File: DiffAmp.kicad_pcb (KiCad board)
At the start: 2 copper layers, 99.7 x 35.6 mm, 111 parts, among them J1 USB_OTG, J2 Screw_Terminal_1x03, J3 Conn_01x02, J4 Conn_01x02, J5 Conn_01x02, U1 SF_IHXXXXS, U2 TPS7A49, U3 TPS7A30, U4 OPA189, U5 AD8421, U6 OPA189, U7 OPA189

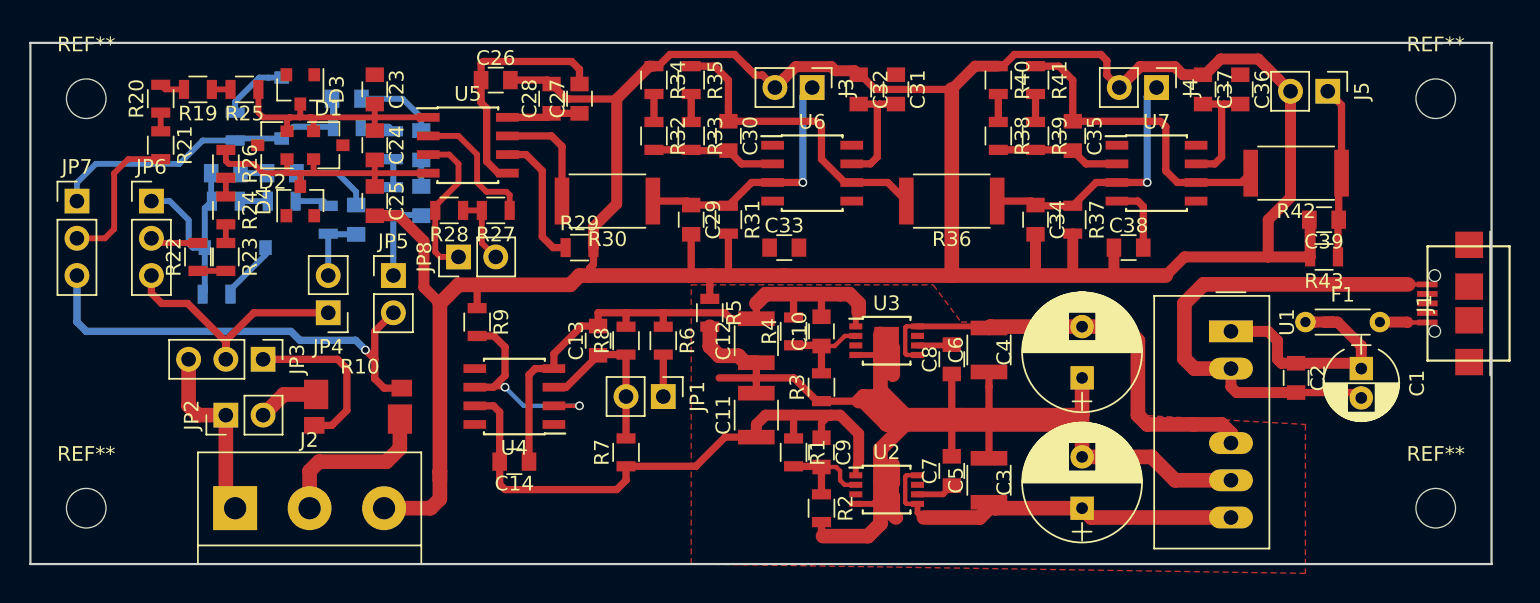
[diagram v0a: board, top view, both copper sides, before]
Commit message: Layout Completed
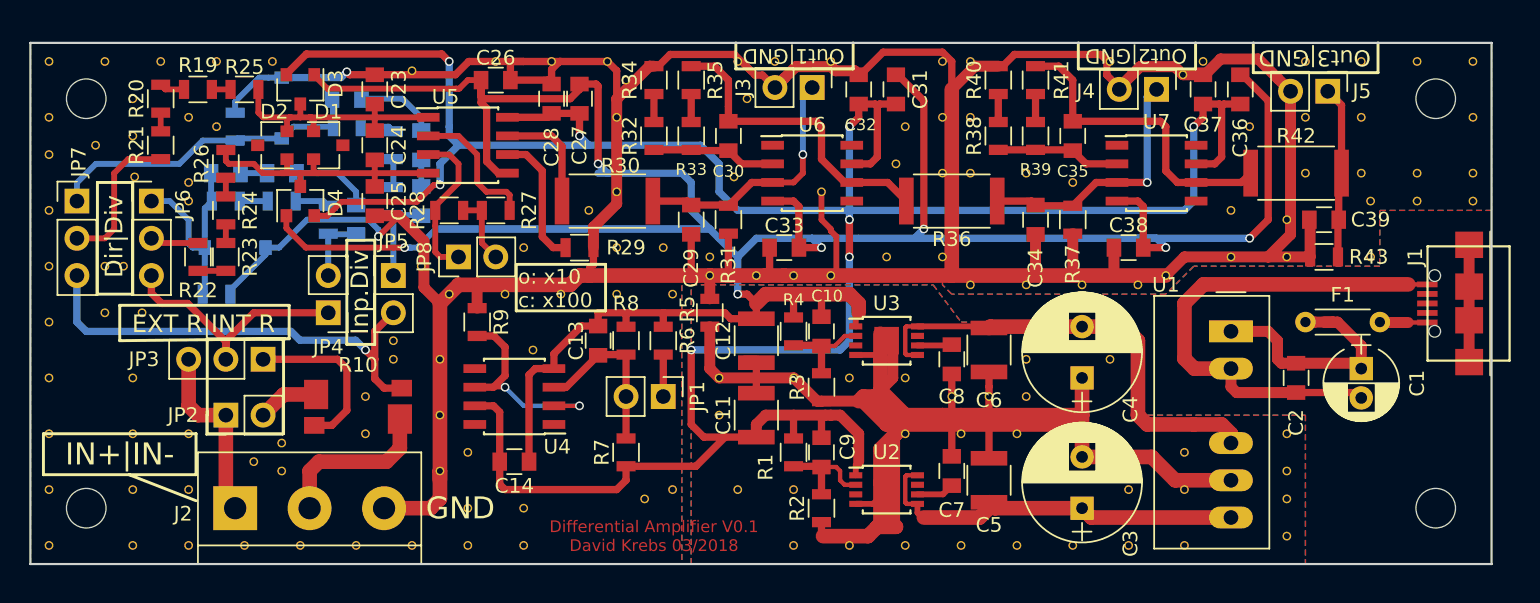
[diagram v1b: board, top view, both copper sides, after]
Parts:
- added ?: , DiffAmp:VIA-0.6mm, F.Cu at (119.8, 68.8)
- added ?: , DiffAmp:VIA-0.6mm, F.Cu at (76.8, 74.9)
- added ?: , DiffAmp:VIA-0.6mm, F.Cu at (162.6, 64.8)
- added ?: , DiffAmp:VIA-0.6mm, F.Cu at (162.6, 68.6)
- added ?: , DiffAmp:VIA-0.6mm, F.Cu at (166.4, 68.6)
- added ?: , DiffAmp:VIA-0.6mm, F.Cu at (170.2, 68.6)
- added ?: , DiffAmp:VIA-0.6mm, F.Cu at (170.2, 64.8)
- added ?: , DiffAmp:VIA-0.6mm, F.Cu at (145.4, 61.0)
- added ?: , DiffAmp:VIA-0.6mm, F.Cu at (134.0, 61.0)
- added ?: , DiffAmp:VIA-0.6mm, F.Cu at (126.4, 61.0)
- added ?: , DiffAmp:VIA-0.6mm, F.Cu at (122.6, 61.0)
- added ?: , DiffAmp:VIA-0.6mm, F.Cu at (103.5, 61.0)
- added ?: , DiffAmp:VIA-0.6mm, F.Cu at (79.4, 78.1)
- added ?: , DiffAmp:VIA-0.6mm, F.Cu at (107.3, 61.0)
- added ?: , DiffAmp:VIA-0.6mm, F.Cu at (111.1, 61.0)
- added ?: , DiffAmp:VIA-0.6mm, F.Cu at (97.8, 61.6)
- added ?: , DiffAmp:VIA-0.6mm, F.Cu at (88.3, 61.0)
- added ?: , DiffAmp:VIA-0.6mm, F.Cu at (84.5, 61.0)
- added ?: , DiffAmp:VIA-0.6mm, F.Cu at (80.6, 61.0)
- added ?: , DiffAmp:VIA-0.6mm, F.Cu at (76.8, 61.0)
- added ?: , DiffAmp:VIA-0.6mm, F.Cu at (73.0, 61.0)
- added ?: , DiffAmp:VIA-0.6mm, F.Cu at (150.4, 61.9)
- added ?: , DiffAmp:VIA-0.6mm, F.Cu at (151.8, 61.0)
- added ?: , DiffAmp:VIA-0.6mm, F.Cu at (76.8, 78.1)
- added ?: , DiffAmp:VIA-0.6mm, F.Cu at (158.8, 61.0)
- added ?: , DiffAmp:VIA-0.6mm, F.Cu at (162.6, 61.0)
- added ?: , DiffAmp:VIA-0.6mm, F.Cu at (166.4, 61.0)
- added ?: , DiffAmp:VIA-0.6mm, F.Cu at (118.7, 85.1)
- added ?: , DiffAmp:VIA-0.6mm, F.Cu at (118.7, 82.5)
- added ?: , DiffAmp:VIA-0.6mm, F.Cu at (123.8, 82.5)
- added ?: , DiffAmp:VIA-0.6mm, F.Cu at (134.6, 83.8)
- added ?: , DiffAmp:VIA-0.6mm, F.Cu at (127.6, 82.5)
- added ?: , DiffAmp:VIA-0.6mm, F.Cu at (131.4, 82.5)
- added ?: , DiffAmp:VIA-0.6mm, F.Cu at (137.2, 83.8)
- added ?: , DiffAmp:VIA-0.6mm, F.Cu at (78.1, 74.9)
- added ?: , DiffAmp:VIA-0.6mm, F.Cu at (139.7, 83.8)
- added ?: , DiffAmp:VIA-0.6mm, F.Cu at (139.7, 81.3)
- added ?: , DiffAmp:VIA-0.6mm, F.Cu at (145.4, 81.3)
- added ? (x2): , DiffAmp:VIA-0.6mm, F.Cu at (142.9, 86.4)
- added ?: , DiffAmp:VIA-0.6mm, F.Cu at (139.1, 86.4)
- added ?: , DiffAmp:VIA-0.6mm, F.Cu at (135.3, 86.4)
- added ?: , DiffAmp:VIA-0.6mm, F.Cu at (131.4, 86.4)
- added ?: , DiffAmp:VIA-0.6mm, F.Cu at (120.0, 90.2)
- added ?: , DiffAmp:VIA-0.6mm, F.Cu at (123.8, 90.2)
- added ?: , DiffAmp:VIA-0.6mm, F.Cu at (78.7, 82.5)
- added ?: , DiffAmp:VIA-0.6mm, F.Cu at (123.8, 94.0)
- added ?: , DiffAmp:VIA-0.6mm, F.Cu at (127.6, 94.0)
- added ?: , DiffAmp:VIA-0.6mm, F.Cu at (131.4, 94.0)
- added ?: , DiffAmp:VIA-0.6mm, F.Cu at (135.3, 94.0)
- added ?: , DiffAmp:VIA-0.6mm, F.Cu at (139.1, 94.0)
- added ?: , DiffAmp:VIA-0.6mm, F.Cu at (142.9, 94.0)
- added ?: , DiffAmp:VIA-0.6mm, F.Cu at (150.5, 94.0)
- added ?: , DiffAmp:VIA-0.6mm, F.Cu at (146.7, 94.0)
- added ?: , DiffAmp:VIA-0.6mm, F.Cu at (146.7, 87.6)
- added ?: , DiffAmp:VIA-0.6mm, F.Cu at (146.7, 90.2)
- added ?: , DiffAmp:VIA-0.6mm, F.Cu at (82.5, 90.2)
- added ?: , DiffAmp:VIA-0.6mm, F.Cu at (150.5, 90.2)
- added ?: , DiffAmp:VIA-0.6mm, F.Cu at (150.5, 87.6)
- added ?: , DiffAmp:VIA-0.6mm, F.Cu at (157.5, 88.9)
- added ?: , DiffAmp:VIA-0.6mm, F.Cu at (157.5, 90.8)
- added ?: , DiffAmp:VIA-0.6mm, F.Cu at (157.5, 93.3)
- added ?: , DiffAmp:VIA-0.6mm, F.Cu at (157.5, 86.4)
- added ?: , DiffAmp:VIA-0.6mm, F.Cu at (170.2, 61.0)
- added ?: , DiffAmp:VIA-0.6mm, F.Cu at (82.5, 86.4)
- added ?: , DiffAmp:VIA-0.6mm, F.Cu at (78.7, 86.4)
- added ?: , DiffAmp:VIA-0.6mm, F.Cu at (78.7, 90.2)
- added ?: , DiffAmp:VIA-0.6mm, F.Cu at (73.0, 64.8)
- added ?: , DiffAmp:VIA-0.6mm, F.Cu at (76.2, 66.7)
- added ?: , DiffAmp:VIA-0.6mm, F.Cu at (73.0, 67.3)
- added ?: , DiffAmp:VIA-0.6mm, F.Cu at (73.0, 71.1)
- added ?: , DiffAmp:VIA-0.6mm, F.Cu at (73.0, 74.9)
- added ?: , DiffAmp:VIA-0.6mm, F.Cu at (73.0, 78.7)
- added ?: , DiffAmp:VIA-0.6mm, F.Cu at (73.0, 82.5)
- added ?: , DiffAmp:VIA-0.6mm, F.Cu at (73.0, 86.4)
- added ?: , DiffAmp:VIA-0.6mm, F.Cu at (73.0, 90.2)
- added ?: , DiffAmp:VIA-0.6mm, F.Cu at (88.9, 88.9)
- added ?: , DiffAmp:VIA-0.6mm, F.Cu at (87.0, 88.3)
- added ?: , DiffAmp:VIA-0.6mm, F.Cu at (88.9, 87.0)
- added ?: , DiffAmp:VIA-0.6mm, F.Cu at (78.7, 63.5)
- added ?: , DiffAmp:VIA-0.6mm, F.Cu at (94.6, 86.4)
- added ?: , DiffAmp:VIA-0.6mm, F.Cu at (94.6, 83.8)
- added ?: , DiffAmp:VIA-0.6mm, F.Cu at (101.6, 87.6)
- added ?: , DiffAmp:VIA-0.6mm, F.Cu at (101.6, 91.4)
- added ?: , DiffAmp:VIA-0.6mm, F.Cu at (105.4, 91.4)
- added ?: , DiffAmp:VIA-0.6mm, F.Cu at (73.0, 94.0)
- added ?: , DiffAmp:VIA-0.6mm, F.Cu at (78.7, 94.0)
- added ?: , DiffAmp:VIA-0.6mm, F.Cu at (82.5, 94.0)
- added ?: , DiffAmp:VIA-0.6mm, F.Cu at (86.4, 94.0)
- added ?: , DiffAmp:VIA-0.6mm, F.Cu at (90.2, 94.0)
- added ?: , DiffAmp:VIA-0.6mm, F.Cu at (78.7, 66.0)
- added ?: , DiffAmp:VIA-0.6mm, F.Cu at (94.0, 94.0)
- added ?: , DiffAmp:VIA-0.6mm, F.Cu at (97.8, 94.0)
- added ?: , DiffAmp:VIA-0.6mm, F.Cu at (101.6, 94.0)
- added ?: , DiffAmp:VIA-0.6mm, F.Cu at (99.7, 88.9)
- added ?: , DiffAmp:VIA-0.6mm, F.Cu at (99.7, 85.1)
- added ?: , DiffAmp:VIA-0.6mm, F.Cu at (99.7, 81.3)
- added ?: , DiffAmp:VIA-0.6mm, F.Cu at (96.5, 81.3)
- added ?: , DiffAmp:VIA-0.6mm, F.Cu at (96.5, 80.0)
- added ?: , DiffAmp:VIA-0.6mm, F.Cu at (98.4, 74.9)
- added ?: , DiffAmp:VIA-0.6mm, F.Cu at (100.3, 76.8)
- added ?: , DiffAmp:VIA-0.6mm, F.Cu at (82.5, 70.5)
- added ?: , DiffAmp:VIA-0.6mm, F.Cu at (105.4, 94.0)
- added ?: , DiffAmp:VIA-0.6mm, F.Cu at (113.7, 90.8)
- added ?: , DiffAmp:VIA-0.6mm, F.Cu at (115.6, 90.2)
- added ?: , DiffAmp:VIA-0.6mm, F.Cu at (106.0, 80.6)
- added ?: , DiffAmp:VIA-0.6mm, F.Cu at (105.4, 73.7)
- added ?: , DiffAmp:VIA-0.6mm, F.Cu at (104.1, 76.8)
- added ?: , DiffAmp:VIA-0.6mm, F.Cu at (108.0, 76.8)
- added ?: , DiffAmp:VIA-0.6mm, F.Cu at (109.9, 71.1)
- added ?: , DiffAmp:VIA-0.6mm, F.Cu at (111.8, 69.8)
- added ?: , DiffAmp:VIA-0.6mm, F.Cu at (112.4, 62.2)
- added ?: , DiffAmp:VIA-0.6mm, F.Cu at (78.9, 68.8)
- added ?: , DiffAmp:VIA-0.6mm, F.Cu at (111.8, 64.8)
- added ?: , DiffAmp:VIA-0.6mm, F.Cu at (120.0, 61.0)
- added ?: , DiffAmp:VIA-0.6mm, F.Cu at (120.7, 63.5)
- added ?: , DiffAmp:VIA-0.6mm, F.Cu at (125.7, 69.8)
- added ?: , DiffAmp:VIA-0.6mm, F.Cu at (111.8, 76.8)
- added ?: , DiffAmp:VIA-0.6mm, F.Cu at (115.6, 76.8)
- added ?: , DiffAmp:VIA-0.6mm, F.Cu at (111.8, 73.7)
- added ?: , DiffAmp:VIA-0.6mm, F.Cu at (114.9, 73.7)
- added ?: , DiffAmp:VIA-0.6mm, F.Cu at (118.1, 74.3)
- added ?: , DiffAmp:VIA-0.6mm, F.Cu at (118.1, 75.6)
- added ?: , DiffAmp:VIA-0.6mm, F.Cu at (82.5, 69.2)
- added ?: , DiffAmp:VIA-0.6mm, F.Cu at (123.8, 75.6)
- added ?: , DiffAmp:VIA-0.6mm, F.Cu at (121.3, 75.6)
- added ?: , DiffAmp:VIA-0.6mm, F.Cu at (126.4, 75.6)
- added ?: , DiffAmp:VIA-0.6mm, F.Cu at (130.8, 67.9)
- added ?: , DiffAmp:VIA-0.6mm, F.Cu at (131.4, 65.4)
- added ?: , DiffAmp:VIA-0.6mm, F.Cu at (154.9, 65.4)
- added ?: , DiffAmp:VIA-0.6mm, F.Cu at (130.2, 74.3)
- added ?: , DiffAmp:VIA-0.6mm, F.Cu at (134.0, 74.3)
- added ?: , DiffAmp:VIA-0.6mm, F.Cu at (134.0, 68.6)
- added ?: , DiffAmp:VIA-0.6mm, F.Cu at (134.0, 64.8)
- added ?: , DiffAmp:VIA-0.6mm, F.Cu at (84.5, 65.4)
- added ?: , DiffAmp:VIA-0.6mm, F.Cu at (135.9, 61.0)
- added ?: , DiffAmp:VIA-0.6mm, F.Cu at (135.9, 64.8)
- added ?: , DiffAmp:VIA-0.6mm, F.Cu at (142.9, 69.2)
- added ?: , DiffAmp:VIA-0.6mm, F.Cu at (139.7, 68.6)
- added ?: , DiffAmp:VIA-0.6mm, F.Cu at (135.9, 68.6)
- added ?: , DiffAmp:VIA-0.6mm, F.Cu at (135.9, 76.2)
- added ?: , DiffAmp:VIA-0.6mm, F.Cu at (139.7, 76.2)
- added ?: , DiffAmp:VIA-0.6mm, F.Cu at (143.5, 76.2)
- added ?: , DiffAmp:VIA-0.6mm, F.Cu at (147.3, 76.2)
- added ?: , DiffAmp:VIA-0.6mm, F.Cu at (149.2, 75.6)
- added ?: , DiffAmp:VIA-0.6mm, F.Cu at (82.5, 64.8)
- added ?: , DiffAmp:VIA-0.6mm, F.Cu at (153.7, 71.1)
- added ?: , DiffAmp:VIA-0.6mm, F.Cu at (153.7, 74.3)
- added ?: , DiffAmp:VIA-0.6mm, F.Cu at (157.5, 71.8)
- added ?: , DiffAmp:VIA-0.6mm, F.Cu at (157.5, 74.3)
- added ?: , DiffAmp:VIA-0.6mm, F.Cu at (158.8, 68.6)
- added ?: , DiffAmp:VIA-0.6mm, F.Cu at (158.8, 64.8)
- added ?: , DiffAmp:VIA-0.6mm, F.Cu at (166.4, 70.5)
- added ?: , DiffAmp:VIA-0.6mm, F.Cu at (170.2, 70.5)
- added ?: , DiffAmp:VIA-0.6mm, F.Cu at (163.2, 70.5)
- added ?: , DiffAmp:VIA-0.6mm, F.Cu at (163.2, 74.3)
- moved J4 0.13 mm to (148.6, 62.9)
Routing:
- net VSSA: track 60.8 -> 199.4 mm, vias 0 -> 7
- net VDDA: track 62.7 -> 191.3 mm, vias 0 -> 8
- net GNDA: track 226.5 -> 278.7 mm, vias 0 -> 2
- net Net-(C11-Pad2): track 104.0 -> 125.2 mm
- net Net-(J1-Pad6): track 0.00 -> 8.00 mm
- added copper zone on B.Cu, net GNDA
- added copper zone on F.Cu, net GNDA
- added copper zone on B.Cu, net Net-(C11-Pad2)
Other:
- board text added: "Differential Amplifier V0.1 David Krebs 03/2018"
- board text added: "Dir|Div"
- board text added: "EXT R|INT R"
- board text added: "GND"
- board text added: "IN+|IN-"
- board text added: "Inp.Div"
- board text added: "Out1|GND"
- board text added: "Out2|GND"
- board text added: "Out3|GND"
- board text added: "o: x10 c: x100"
